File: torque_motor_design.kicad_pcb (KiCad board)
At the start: 2 copper layers, 27.9 x 37 mm, 38 parts, among them U1 ATtiny85-20S, U2 OPAMP, U3 OPAMP, U4 L78L05_SO8

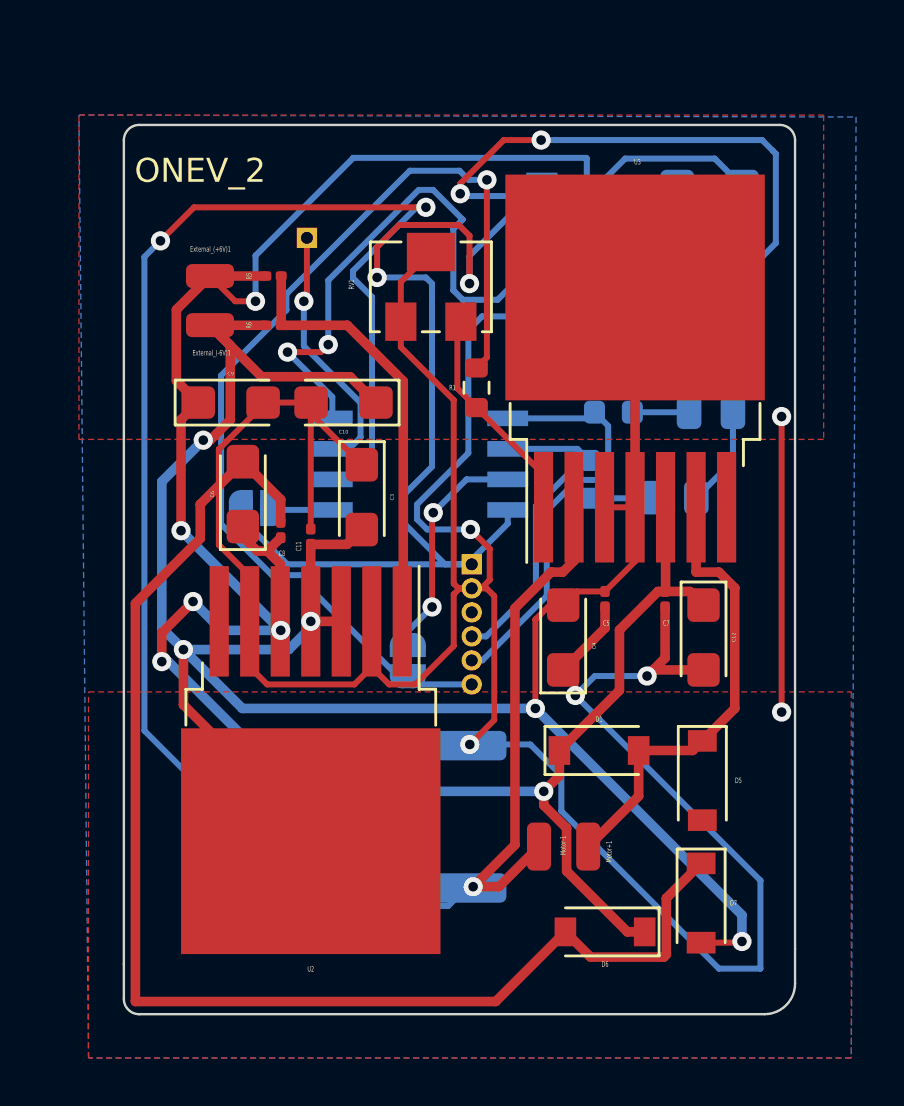
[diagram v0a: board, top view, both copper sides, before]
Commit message: Add:v1.1
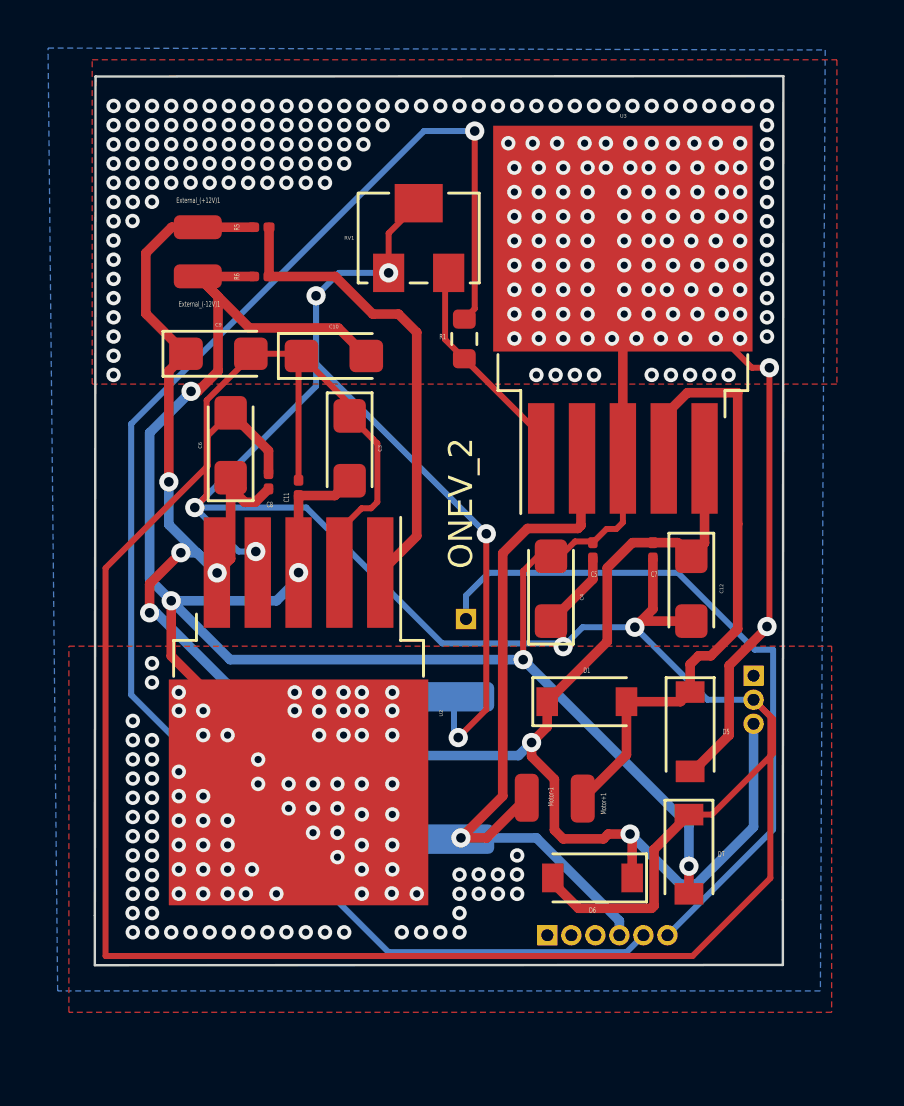
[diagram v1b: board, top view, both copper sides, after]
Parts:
- removed C1, C2: 10uF, Capacitor_Tantalum_SMD:CP_EIA-3216-18_Kemet-A
- removed D3, D4: LED, LED_SMD:LED_0603_1608Metric
- removed Enable_Current_sense, JP1, Torque_mode_EN: Jumper_2_Open, Jumper:SolderJumper-2_P1.3mm_Open_RoundedPad1.0x1.5mm
- removed ONEV_2: PinHeader_1x06_P1.00mm_Vertical, Connector_PinHeader_1.00mm:PinHeader_1x06_P1.00mm_Vertical
- removed R7, R8: 220, Resistor_SMD:R_0805_2012Metric
- removed U1: ATtiny85-20S, Package_SO:SOIC-8W_5.3x5.3mm_P1.27mm
- removed U4: L78L05_SO8, Package_TO_SOT_SMD:SOT-89-3
- added header: PinHeader_1x06_P1.00mm_Vertical, Connector_PinHeader_1.00mm:PinHeader_1x06_P1.00mm_Vertical, B.Cu at (190.3, 69.3)
- added header_2: PinHeader_1x03_P1.00mm_Vertical, Connector_PinHeader_1.00mm:PinHeader_1x03_P1.00mm_Vertical, B.Cu at (198.9, 58.5)
- R1: value 100k -> 49k
- RV1: footprint Potentiometer_SMD:Potentiometer_Bourns_3214W_Vertical -> Potentiometer_SMD:Potentiometer_Bourns_3224W_Vertical
- U2, U3: footprint Package_TO_SOT_SMD:TO-263-7_TabPin8 -> Package_TO_SOT_SMD:TO-263-5_TabPin6
- moved Current_Sense 17.2 mm to (187.0, 56.1)
- moved D6 2.31 mm to (192.2, 66.9)
- moved C11 2.09 mm to (180.0, 50.7)
- moved C3 2.09 mm to (182.1, 49.0)
- moved C4 2.09 mm to (190.5, 54.9)
- moved C8 2.09 mm to (178.7, 50.4)
- moved D1 2.09 mm to (192.0, 59.6)
- moved D5 2.09 mm to (196.3, 60.8)
- moved External_(+12V)1 2.09 mm to (175.8, 39.8)
- moved U3 2.09 mm to (193.5, 43.7)
- moved C12 2.09 mm to (196.3, 54.9)
- moved C5 2.09 mm to (192.2, 53.3)
- moved C6 2.09 mm to (177.2, 48.9)
- moved C7 2.09 mm to (194.7, 53.3)
- moved D7 2.09 mm to (196.2, 65.9)
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- renumbered External_(+6V)1 to External_(+12V)1, External_(-6V)1 to External_(-12V)1
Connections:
- C10 pad 1: -V -> GND
- C10 pad 2: GND -> -V
- R1 pad 1: Torque_mode_jumper -> Torque_Mode
- U2 pad 4: -V -> GND
- U2 pad 6: GND -> -V
- U3 pad 4: -V -> Net-(D1-Pad2)
- U3 pad 6: Net-(D1-Pad2) -> -V
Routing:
- net VCC_MCU_5V: track 77.6 -> 0.00 mm, vias 4 -> 0
- net unconnected-(U1-Pad2): track 56.7 -> 0.00 mm, vias 2 -> 0
- net Torque_Mode: track 9.62 -> 64.7 mm, vias 2 -> 1
- net Torque_mode_jumper: track 42.9 -> 0.00 mm, vias 1 -> 0
- net GND: track 215.7 -> 190.3 mm, vias 6 -> 8
- net +V: track 108.7 -> 88.5 mm
- net current_sense: track 10.7 -> 29.2 mm, vias 1 -> 0
- net TX_Serial: track 17.4 -> 0.00 mm
- net RX_Serial: track 13.5 -> 0.00 mm
- net -V: track 115.4 -> 123.9 mm, vias 7 -> 330
- net Net-(D1-Pad2): track 19.2 -> 26.4 mm
- net Net-(Motor-1-Pad1): track 26.4 -> 31.5 mm
- net Net-(D4-Pad2): track 2.65 -> 0.00 mm
- net Net-(JP1-Pad1): track 2.54 -> 0.00 mm
- net Net-(D3-Pad2): track 2.36 -> 0.00 mm
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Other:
- board size 27.9 x 37 mm -> 28.7 x 37 mm
- board text removed: "5V_MCU"
- board text removed: "GND"
- board text removed: "RX"
- board text removed: "TX"
- board text removed: "Torque"
- board text removed: "Un-Connected"
